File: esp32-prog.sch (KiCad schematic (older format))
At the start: 16 parts, among them J1 USB_C_Receptacle_USB2.0, J2 ESP_PROG, J3 POWER, J4 DTR_RTS, Q1 S8050, Q2 S8050, U1 CH340B, U2 AP1117-33

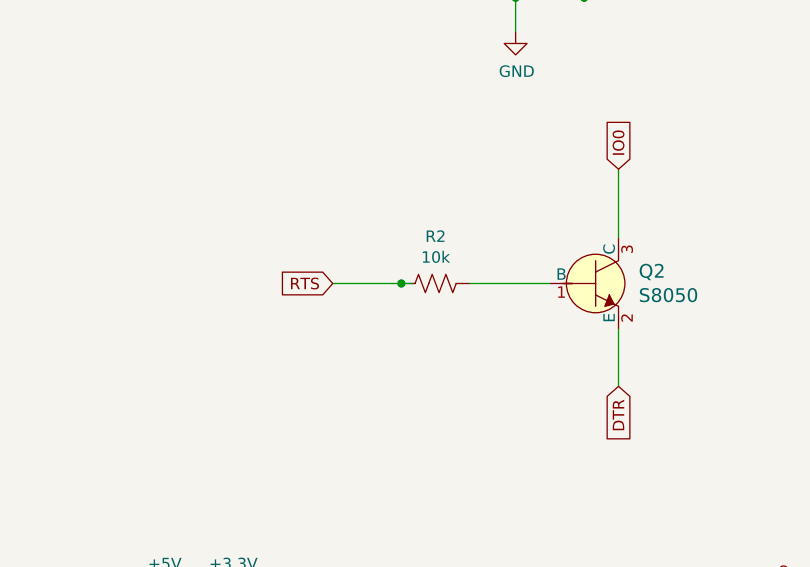
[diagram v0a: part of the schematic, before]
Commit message: Finalise Rev 1.2
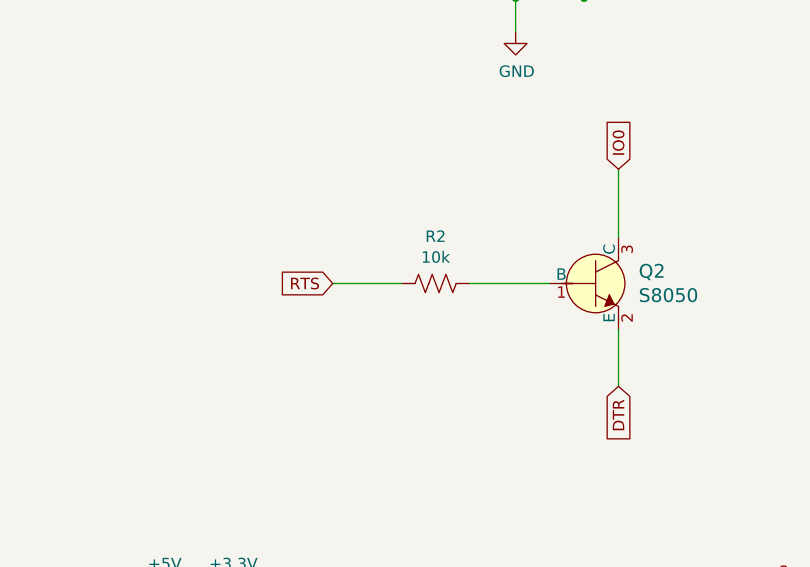
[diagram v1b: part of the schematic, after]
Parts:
- C1, C2: LCSC (none) -> C314285
- C3, C4: LCSC (none) -> C15850
- J1: LCSC (none) -> C165948
- Q1, Q2: LCSC (none) -> C402279
- R1, R2: LCSC (none) -> C169071
- R3, R4: LCSC (none) -> C204553
- U1: LCSC (none) -> C81010
- U2: LCSC (none) -> C351784
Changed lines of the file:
@@
 F 11 "Micro Commercial Co" H 3450 5150 60  0001 L CNN "Manufacturer"
 F 12 "Active" H 3450 5250 60  0001 L CNN "Status"
+F 13 "C402279" H 3250 4050 50  0001 C CNN "LCSC"
 	1    3250 4050
 	1    0    0    -1
@@
 F 2 "Package_SO:SO-16_3.9x9.9mm_P1.27mm" H 2850 2500 50  0001 C CNN
 F 3 "https://datasheet.lcsc.com/szlcsc/2008191806_WCH-Jiangsu-Qin-Heng-CH340B_C81010.pdf" H 2850 2500 50  0001 C CNN
+F 4 "C81010" H 3050 1900 50  0001 C CNN "LCSC"
 	1    3050 1900
 	1    0    0    -1
@@
 F 11 "Micro Commercial Co" H 6700 5200 60  0001 L CNN "Manufacturer"
 F 12 "Active" H 6700 5300 60  0001 L CNN "Status"
+F 13 "C402279" H 6500 4100 50  0001 C CNN "LCSC"
 	1    6500 4100
 	1    0    0    -1
@@
 F 2 "Resistor_SMD:R_0805_2012Metric_Pad1.20x1.40mm_HandSolder" V 2540 4040 50  0001 C CNN
 F 3 "~" H 2500 4050 50  0001 C CNN
+F 4 "C169071" H 2500 4050 50  0001 C CNN "LCSC"
 	1    2500 4050
-	0    1    1    0
-$EndComp
-$Comp
-L Device:R_US R2
-U 1 1 5FD4B2FA
-P 5800 4100
-F 0 "R2" V 5595 4100 50  0000 C CNN
-F 1 "10k" V 5686 4100 50  0000 C CNN
-F 2 "Resistor_SMD:R_0805_2012Metric_Pad1.20x1.40mm_HandSolder" V 5840 4090 50  0001 C CNN
-F 3 "~" H 5800 4100 50  0001 C CNN
-	1    5800 4100
 	0    1    1    0
 $EndComp
@@
 Text GLabel 5350 4100 0    50   Input ~ 0
 RTS
-Wire Wire Line
-	5350 4100 5650 4100
 Wire Wire Line
 	1950 4050 2350 4050
@@
 F 2 "Capacitor_SMD:C_0805_2012Metric_Pad1.18x1.45mm_HandSolder" H 1688 1550 50  0001 C CNN
 F 3 "~" H 1650 1700 50  0001 C CNN
+F 4 "C314285" H 1650 1700 50  0001 C CNN "LCSC"
 	1    1650 1700
 	1    0    0    -1
@@
 F 2 "Capacitor_SMD:C_0805_2012Metric_Pad1.18x1.45mm_HandSolder" H 4188 1550 50  0001 C CNN
 F 3 "~" H 4150 1700 50  0001 C CNN
+F 4 "C314285" H 4150 1700 50  0001 C CNN "LCSC"
 	1    4150 1700
 	1    0    0    -1
@@
 F 2 "Connector_USB:USB_C_Receptacle_HRO_TYPE-C-31-M-12" H 6600 1800 50  0001 C CNN
 F 3 "https://www.usb.org/sites/default/files/documents/usb_type-c.zip" H 6600 1800 50  0001 C CNN
+F 4 "C165948" H 6450 1800 50  0001 C CNN "LCSC"
 	1    6450 1800
 	1    0    0    -1
@@
 F 2 "Resistor_SMD:R_0805_2012Metric_Pad1.20x1.40mm_HandSolder" V 7890 1690 50  0001 C CNN
 F 3 "~" H 7850 1700 50  0001 C CNN
+F 4 "C204553" H 7850 1700 50  0001 C CNN "LCSC"
 	1    7850 1700
 	1    0    0    -1
@@
 F 2 "Resistor_SMD:R_0805_2012Metric_Pad1.20x1.40mm_HandSolder" V 8340 1690 50  0001 C CNN
 F 3 "~" H 8300 1700 50  0001 C CNN
+F 4 "C204553" H 8300 1700 50  0001 C CNN "LCSC"
 	1    8300 1700
 	1    0    0    -1
@@
 F 2 "Package_TO_SOT_SMD:SOT-223-3_TabPin2" H 9100 4300 50  0001 C CNN
 F 3 "http://www.diodes.com/datasheets/AP1117.pdf" H 9200 3850 50  0001 C CNN
+F 4 "C351784" H 9100 4100 50  0001 C CNN "LCSC"
 	1    9100 4100
 	1    0    0    -1
@@
 F 2 "Capacitor_SMD:C_0805_2012Metric_Pad1.18x1.45mm_HandSolder" H 8338 4100 50  0001 C CNN
 F 3 "~" H 8300 4250 50  0001 C CNN
+F 4 "C15850" H 8300 4250 50  0001 C CNN "LCSC"
 	1    8300 4250
 	1    0    0    -1
@@
 F 2 "Capacitor_SMD:C_0805_2012Metric_Pad1.18x1.45mm_HandSolder" H 9838 4100 50  0001 C CNN
 F 3 "~" H 9800 4250 50  0001 C CNN
+F 4 "C15850" H 9800 4250 50  0001 C CNN "LCSC"
 	1    9800 4250
 	1    0    0    -1
@@
 Wire Wire Line
 	4900 6250 4900 6600
-Connection ~ 5650 4100
-Wire Wire Line
-	5650 4100 5700 4100
-Wire Wire Line
-	5950 4100 6300 4100
 NoConn ~ 3400 1650
 NoConn ~ 3400 1950
@@
 Wire Wire Line
 	7250 5500 7050 5500
+Wire Wire Line
+	5950 4100 6300 4100
+$Comp
+L Device:R_US R2
+U 1 1 5FD4B2FA
+P 5800 4100
+F 0 "R2" V 5595 4100 50  0000 C CNN
+F 1 "10k" V 5686 4100 50  0000 C CNN
+F 2 "Resistor_SMD:R_0805_2012Metric_Pad1.20x1.40mm_HandSolder" V 5840 4090 50  0001 C CNN
+F 3 "~" H 5800 4100 50  0001 C CNN
+F 4 "C169071" H 5800 4100 50  0001 C CNN "LCSC"
+	1    5800 4100
+	0    1    1    0
+$EndComp
+Wire Wire Line
+	5350 4100 5650 4100
 $EndSCHEMATC
